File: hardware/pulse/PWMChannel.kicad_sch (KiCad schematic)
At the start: 6 parts, among them J201 WAGO-2065, J202 WAGO-2065, Q201 BSC010N04LS

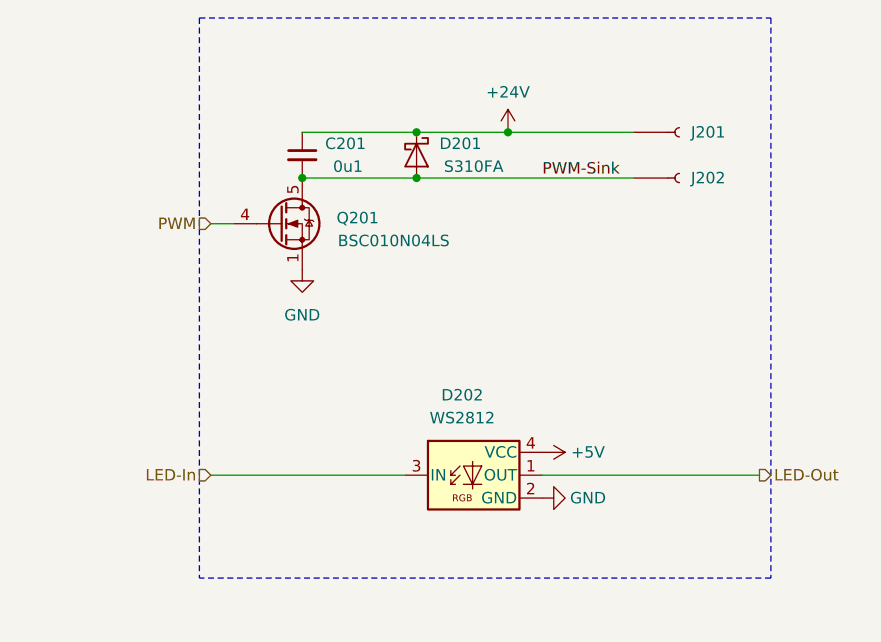
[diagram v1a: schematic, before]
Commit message: Update parts
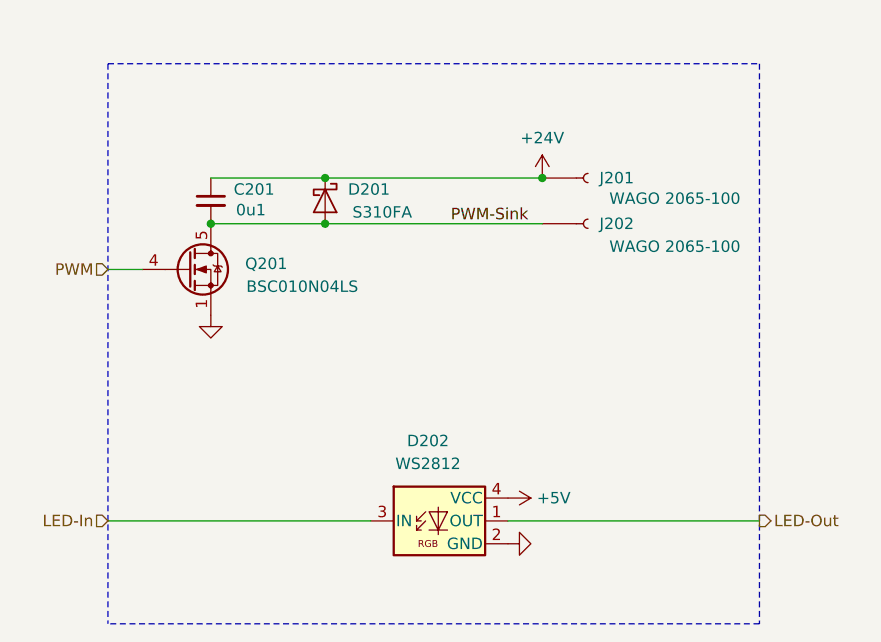
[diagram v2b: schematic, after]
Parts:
- C201: footprint Capacitor_SMD:C_0603_1608Metric -> V2_Capacitor_SMD:C_0603; symbol Device:C_Small -> V2_Device:C_0603_0u1; Manufacturer (none) -> TDK; Mouser (none) -> 810-CGA3E2X7R1H104MA; Product (none) -> CGA3E2X7R1H104M080AA
- D201: footprint Diode_SMD:D_SOD-123F -> V2_Diode_SMD:D_SOD-123F; Manufacturer (none) -> onsemi; Mouser (none) -> 512-S310FA; Product (none) -> S310FA
- D202: LCSC (none) -> C965555; Manufacturer (none) -> Worldsemi; Product (none) -> WS2812B-2020
- J201, J202: value WAGO-2065 -> WAGO 2065-100; Manufacturer (none) -> WAGO; Product (none) -> 2065-100/998-403
- Q201: Manufacturer (none) -> Infineon Technologies; Mouser (none) -> 726-BSC010N04LS; Product (none) -> BSC010N04LS
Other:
- moved on the sheet: C201, D201, D202, J201, J202, Q201

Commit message: Refresh
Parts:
- Q201: Polarity (none) -> N; Rating (none) -> 40V
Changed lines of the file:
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@@
-			)
-		)
-		(property "Sim.Pin" ""
-			(at 135.89 93.98 90)
-			(effects
-				(font
-					(size 1.27 1.27)
-				)
-				(hide yes)
 			)
 		)
@@
 		(property "Product" "S310FA"
 			(at 123.19 93.98 0)
-			(effects
-				(font
-					(size 1.27 1.27)
-				)
-				(hide yes)
-			)
-		)
-		(property "Sim.Enable" ""
-			(at 135.89 93.98 90)
 			(effects
 				(font
@@
 			)
 		)
-		(property "Sim.Pin" ""
-			(at 123.19 93.98 0)
-			(effects
-				(font
-					(size 1.27 1.27)
-				)
-				(hide yes)
-			)
-		)
 		(property "Manufacturer" "TDK"
 			(at 123.19 109.22 0)
@@
 		(property "Product" "CGA3E2X7R1H104M080AA"
 			(at 123.19 111.76 0)
-			(effects
-				(font
-					(size 1.27 1.27)
-				)
-				(hide yes)
-			)
-		)
-		(property "Sim.Enable" ""
-			(at 123.19 93.98 0)
 			(effects
 				(font
@@
 			)
 		)
-		(property "Sim.Pin" ""
-			(at 120.65 101.6 0)
-			(effects
-				(font
-					(size 1.27 1.27)
-				)
-				(hide yes)
-			)
-		)
 		(property "Product" "BSC010N04LS"
 			(at 120.65 121.92 0)
@@
 			)
 		)
-		(property "Sim.Enable" ""
-			(at 120.65 101.6 0)
+		(property "Rating" "40V"
+			(at 120.65 121.92 0)
+			(effects
+				(font
+					(size 1.27 1.27)
+				)
+				(hide yes)
+			)
+		)
+		(property "Polarity" "N"
+			(at 120.65 119.38 0)
 			(effects
 				(font
@@
 			)
 		)
-		(property "Sim.Pin" ""
-			(at 148.59 130.81 0)
-			(effects
-				(font
-					(size 1.27 1.27)
-				)
-				(hide yes)
-			)
-		)
-		(property "Sim.Enable" ""
-			(at 148.59 130.81 0)
-			(effects
-				(font
-					(size 1.27 1.27)
-				)
-				(hide yes)
-			)
-		)
 		(pin "1"
 		)
@@
 			)
 		)
-		(property "Sim.Pin" ""
-			(at 165.1 91.44 0)
-			(effects
-				(font
-					(size 1.27 1.27)
-				)
-				(hide yes)
-			)
-		)
-		(property "Sim.Enable" ""
-			(at 165.1 91.44 0)
-			(effects
-				(font
-					(size 1.27 1.27)
-				)
-				(hide yes)
-			)
-		)
 		(pin "1"
 		)
@@
 			(effects
 				(font
-					(size 1.27 1.27)
-				)
-				(hide yes)
-			)
-		)
-		(property "Sim.Pin" ""
-			(at 165.1 96.52 0)
-			(effects
-				(font
-					(size 1.27 1.27)
-				)
-				(hide yes)
-			)
-		)
-		(property "Sim.Enable" ""
-			(at 165.1 96.52 0)
-			(effects
-				(font
